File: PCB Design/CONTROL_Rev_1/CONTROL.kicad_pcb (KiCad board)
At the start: 2 copper layers, 40 x 80 mm, 50 parts, among them J1 Conn_01x24_Pin, J2 Conn_01x24_Pin, J3 Micro_SD_Card, J4 USB_C_Receptacle_USB2.0_16P, SW1 SW_SPDT, U1 STM32F446RET6, U2 USBLC6-2SC6, Y1 16MHz, Y2 32.768KHz

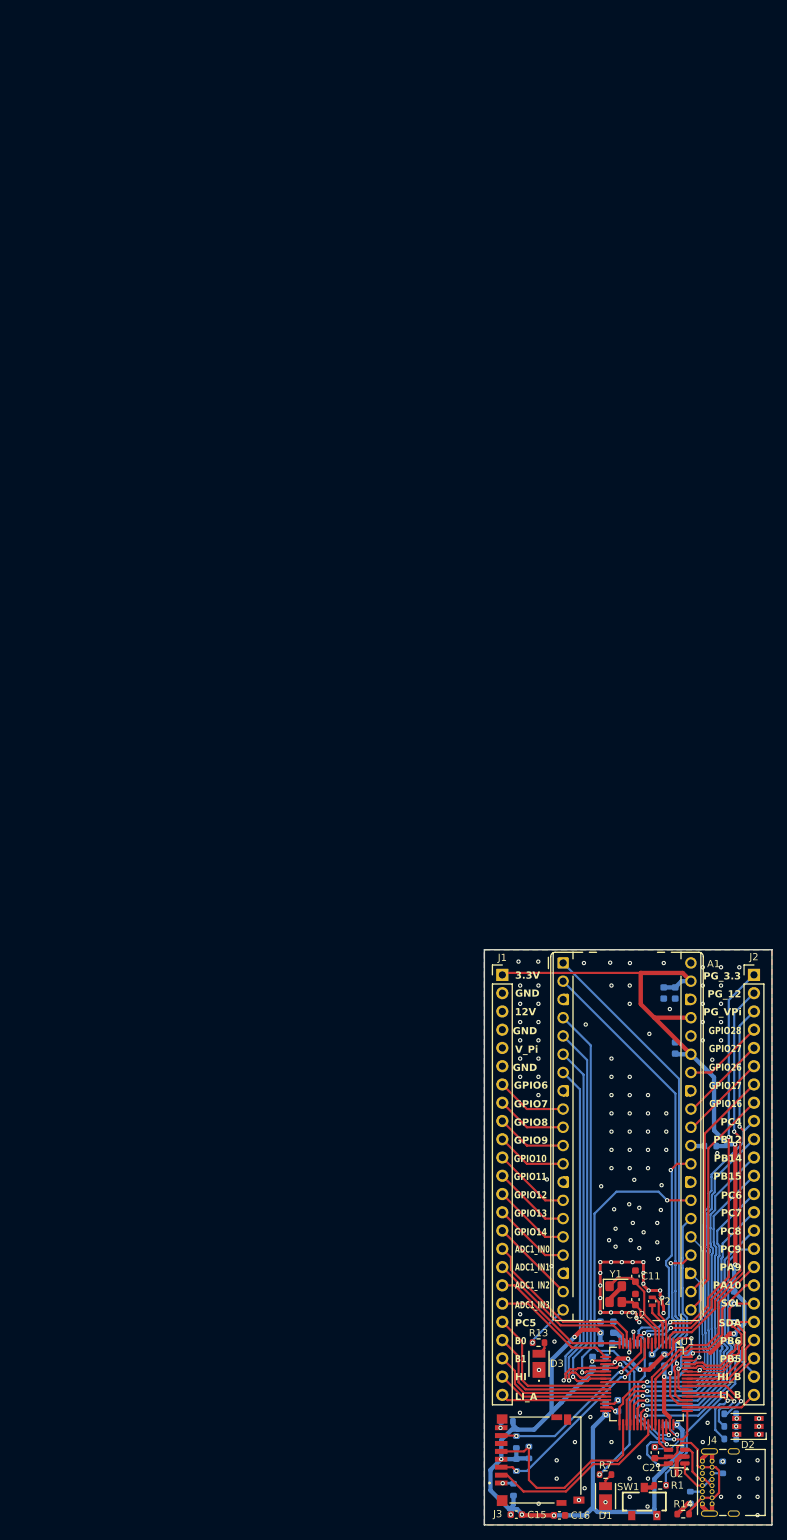
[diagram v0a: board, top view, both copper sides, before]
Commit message: Updated
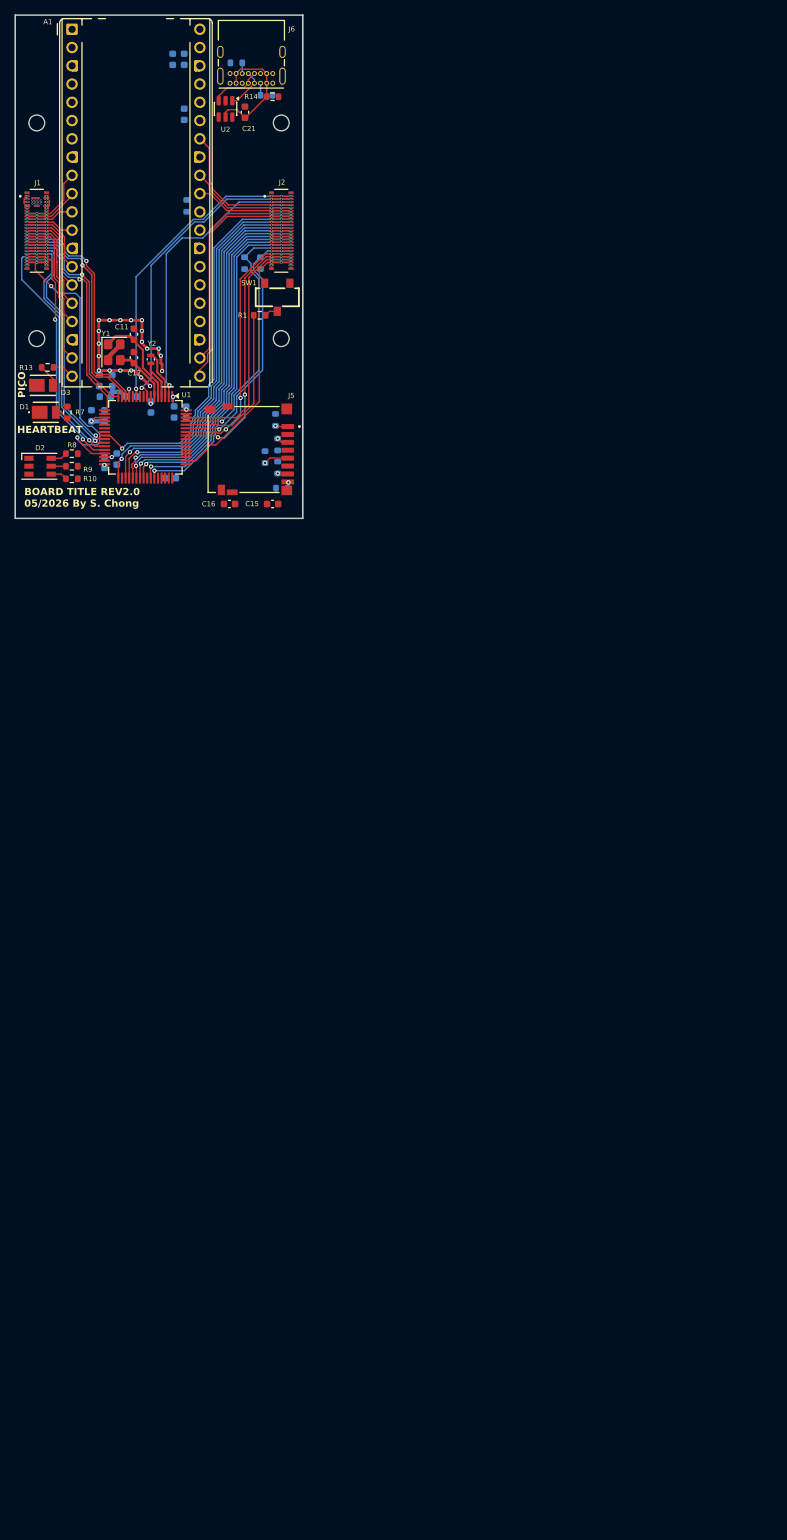
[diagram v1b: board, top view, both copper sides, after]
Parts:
- added J5: Micro_SD_Card, CONTROL:AMPHENOL_1140084168, F.Cu at (17.0, 30.4)
- added J6: USB_C_Receptacle_USB2.0_16P, Connector_USB:USB_C_Receptacle_GCT_USB4085, F.Cu at (15.8, -20.5)
- added REF**: MountingHole_2.2mm_M2, MountingHole:MountingHole_2.2mm_M2, F.Cu at (-17.0, 15.0)
- added REF**: MountingHole_2.2mm_M2, MountingHole:MountingHole_2.2mm_M2, F.Cu at (17.0, 15.0)
- added REF**: MountingHole_2.2mm_M2, MountingHole:MountingHole_2.2mm_M2, F.Cu at (-17.0, -15.0)
- added REF**: MountingHole_2.2mm_M2, MountingHole:MountingHole_2.2mm_M2, F.Cu at (17.0, -15.0)
- J1, J2: value Conn_01x24_Pin -> Conn_02x25_Odd_Even; footprint Connector_PinHeader_2.54mm:PinHeader_1x24_P2.54mm_Vertical -> CONTROL:HIROSE_DF40C-50DP-0.4V_51_
- J3: value Micro_SD_Card -> Conn_02x25_Odd_Even; footprint CONTROL:AMPHENOL_1140084168 -> CONTROL:HIROSE_DF40C-50DP-0.4V_51_; moved to B.Cu
- J4: value USB_C_Receptacle_USB2.0_16P -> Conn_02x25_Odd_Even; footprint Connector_USB:USB_C_Receptacle_GCT_USB4085 -> CONTROL:HIROSE_DF40C-50DP-0.4V_51_; moved to B.Cu
- R10, R8, R9: moved to F.Cu
- moved R12 206.7 mm to (10.8, -23.4), turned to 180 degrees
- moved R14 205.3 mm to (15.8, -18.6), turned to 0 degrees
- moved R11 203.8 mm to (14.9, -18.9), turned to 0 degrees
- moved U2 197.7 mm to (9.25, -16.9), turned to -90 degrees
- moved C21 195.0 mm to (11.9, -16.5)
- moved J4 186.5 mm to (17.0, 0.00), turned to -90 degrees
- moved J3 183.1 mm to (-17.0, 0.00)
- moved SW1 175.1 mm to (16.4, 9.25), turned to 180 degrees
- moved R1 172.0 mm to (14.0, 11.8), turned to 180 degrees
- moved D1 169.7 mm to (-15.8, 25.2), turned to 180 degrees
- moved D2 165.9 mm to (-16.6, 32.8), turned to 0 degrees
- moved R7 165.6 mm to (-12.8, 25.2), turned to 90 degrees
- moved R8 164.8 mm to (-12.1, 31.0), turned to 0 degrees
- moved R3 162.1 mm to (14.1, 4.50)
- moved R9 161.9 mm to (-12.1, 32.8), turned to 0 degrees
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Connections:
- J1 pad 1: 3.3V -> GND
- J1 pad 10: /GPIO_9 -> GND
- J1 pad 11: /GPIO_10 -> GND
- J1 pad 12: /GPIO_11 -> GND
- J1 pad 13: /GPIO_12 -> /GPIO_6
- J1 pad 14: /GPIO_13 -> /GPIO_6
- J1 pad 15: /GPIO_14 -> /GPIO_7
- J1 pad 16: /ADC1_IN0 -> /GPIO_7
- J1 pad 17: /ADC1_IN1 -> /GPIO_8
- J1 pad 18: /ADC1_IN2 -> /GPIO_8
- J1 pad 19: /ADC1_IN3 -> /GPIO_9
- J1 pad 20: /PC5 -> /GPIO_9
- J1 pad 21: /PB0 -> /GPIO_10
- J1 pad 22: /PB1 -> /GPIO_10
- J1 pad 23: /HI_A -> /GPIO_11
- J1 pad 24: /LI_A -> /GPIO_11
- J1 pad 3: 12V -> 3.3V
- J1 pad 4: GND -> 3.3V
- J1 pad 5: V_Piezo -> 3.3V
- J1 pad 6: GND -> 3.3V
- J1 pad 7: /GPIO_6 -> 3.3V
- J1 pad 8: /GPIO_7 -> 3.3V
- J1 pad 9: /GPIO_8 -> GND
- J2 pad 10: /PB12 -> /GPIO_27
- J2 pad 11: /PB14 -> /GPIO_26
- J2 pad 12: /PB15 -> /GPIO_26
- J2 pad 13: /PC6 -> /GPIO_17
- J2 pad 14: /PC7 -> /GPIO_17
- J2 pad 15: /PC8 -> /GPIO_16
- J2 pad 16: /PC9 -> /GPIO_16
- J2 pad 17: /PA9 -> /PC4
- J2 pad 18: /PA10 -> /PC4
- J2 pad 19: /SCL -> /PB12
- J2 pad 2: /PC0 -> /PC3
- J2 pad 20: /SDA -> /PB12
- J2 pad 21: /PB6 -> /PB14
- J2 pad 22: /PB5 -> /PB14
- J2 pad 23: /HI_B -> /PB15
- J2 pad 24: /LI_B -> /PB15
- J2 pad 3: /PC13 -> /PC0
- J2 pad 4: /GPIO_28 -> /PC0
- J2 pad 5: /GPIO_27 -> /PC13
- J2 pad 6: /GPIO_26 -> /PC13
- J2 pad 7: /GPIO_17 -> /GPIO_28
- J2 pad 8: /GPIO_16 -> /GPIO_28
- J2 pad 9: /PC4 -> /GPIO_27
- J3 pad 1: /DAT2 -> GND
- J3 pad 10: (no net) -> GND
- J3 pad 2: /CS -> GND
- J3 pad 3: /SPI2_MOSI -> 3.3V
- J3 pad 5: /SPI2_SCK -> 3.3V
- J3 pad 6: GND -> 3.3V
- J3 pad 7: /SPI2_MISO -> 3.3V
- J3 pad 8: /DAT1 -> 3.3V
- R11 pad 1: Net-(J4-CC1) -> Net-(J6-CC1)
- R12 pad 1: Net-(J4-CC2) -> Net-(J6-CC2)
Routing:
- net 3.3V: track 246.4 -> 6.47 mm, vias 17 -> 18
- net /HEARTBEAT: track 71.6 -> 0.00 mm, vias 3 -> 0
- net /STM_UART_RX: track 69.8 -> 0.00 mm, vias 1 -> 0
- net /STM_UART_TX: track 67.8 -> 0.00 mm, vias 1 -> 0
- net /SWCLK: track 59.1 -> 0.00 mm, vias 2 -> 0
- net GND: track 89.5 -> 33.1 mm, vias 139 -> 30
- net /SPI_SCK: track 54.8 -> 0.00 mm, vias 1 -> 0
- net /SPI_MOSI: track 54.5 -> 0.00 mm, vias 1 -> 0
- net /SPI_MISO: track 53.9 -> 0.00 mm, vias 1 -> 0
- net /SWDIO: track 48.6 -> 0.00 mm, vias 2 -> 0
- net /LI_A: track 14.7 -> 44.6 mm, vias 0 -> 5
- net /LI_B: track 9.99 -> 39.4 mm, vias 0 -> 3
- net /PB5: track 10.6 -> 39.0 mm, vias 0 -> 5
- net /SPI2_MOSI: track 28.7 -> 2.32 mm, vias 2 -> 1
- net /PB6: track 12.5 -> 38.9 mm, vias 0 -> 5
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- added copper zone on B.Cu, net 3.3V
- added copper zone on F.Cu, net 3.3V
- removed copper zone on B.Cu, net GND
- removed copper zone on F.Cu, net GND
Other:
- board size 40 x 80 mm -> 40 x 70 mm
- board text added: "BOARD TITLE REV2.0 05/2026 By S. Chong"
- board text added: "HEARTBEAT"
- board text added: "PICO"
- board text removed: "12V"
- board text removed: "3.3V"
- board text removed: "ADC1_IN0"
- board text removed: "ADC1_IN1"
- board text removed: "ADC1_IN2"
- board text removed: "ADC1_IN3"
- board text removed: "B0"
- board text removed: "B1"
- board text removed: "CONTROL BOARD REV1.1 03/2026 By Samantha Chong"
- board text removed: "GND"
- board text removed: "GPIO10"
- board text removed: "GPIO11"
- board text removed: "GPIO12"
- board text removed: "GPIO13"
- board text removed: "GPIO14"
- board text removed: "GPIO16"
- board text removed: "GPIO17"
- board text removed: "GPIO26"
- board text removed: "GPIO27"
- board text removed: "GPIO28"
- board text removed: "GPIO6"
- board text removed: "GPIO7"
- board text removed: "GPIO8"
- board text removed: "GPIO9"
- board text removed: "HI"
- board text removed: "HI_B"
- board text removed: "LI_A"
- board text removed: "LI_B"
- board text removed: "PA10"
- board text removed: "PA9"
- board text removed: "PB12"
- board text removed: "PB14"
- board text removed: "PB15"
- board text removed: "PB5"
- board text removed: "PB6"
- board text removed: "PC4"
- board text removed: "PC5"
- board text removed: "PC6"
- board text removed: "PC7"
- board text removed: "PC8"
- board text removed: "PC9"
- board text removed: "PG_12"
- board text removed: "PG_3.3"
- board text removed: "PG_VPi"
- board text removed: "SCL"
- board text removed: "SDA"
- board text removed: "V_Pi"

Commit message: Revert "Updated"
This reverts commit 89be44ed720659141c8ee702c54a520a60db740f.
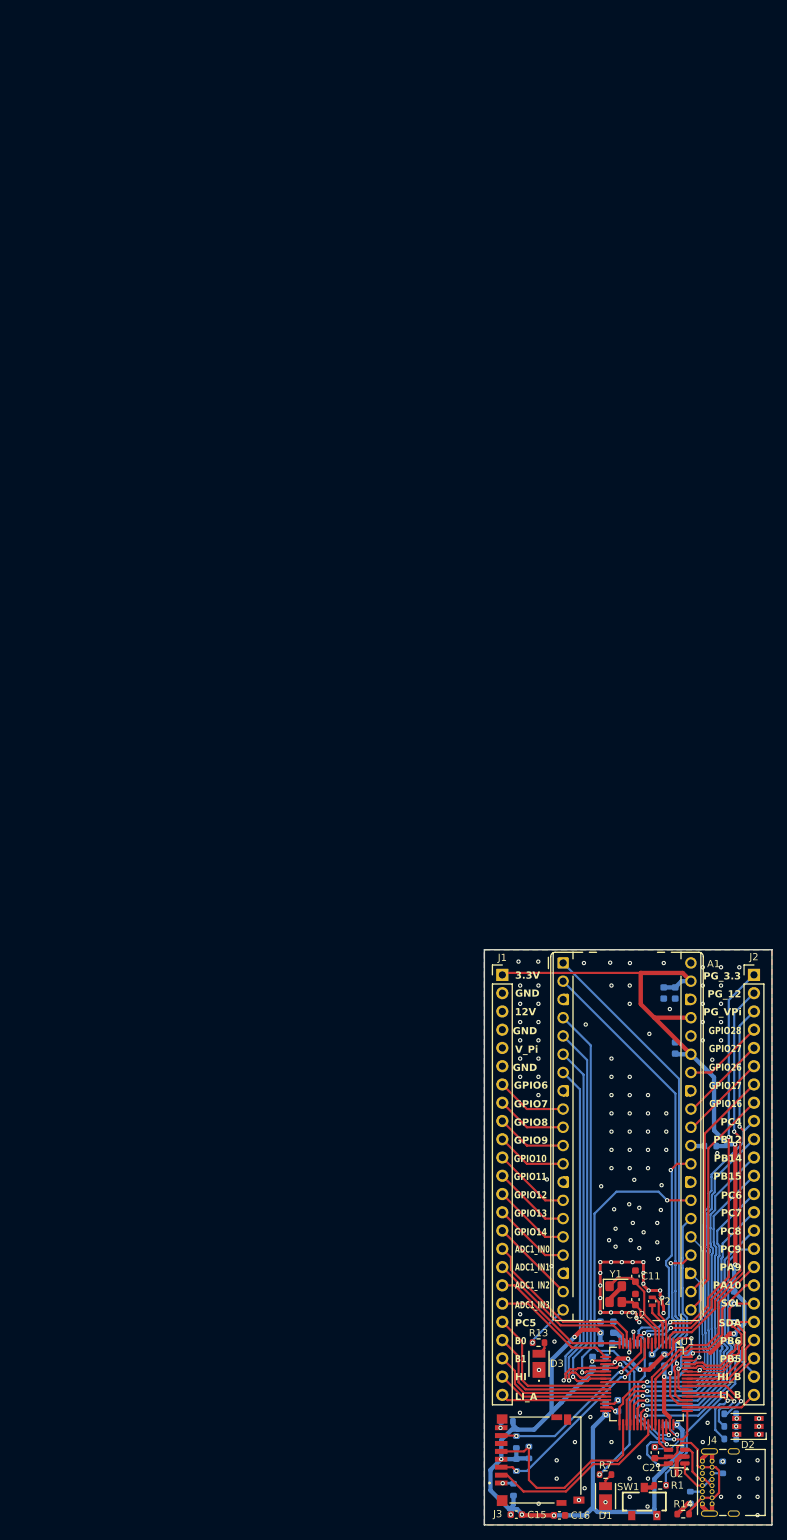
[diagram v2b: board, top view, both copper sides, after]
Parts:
- removed J5: Micro_SD_Card, CONTROL:AMPHENOL_1140084168
- removed J6: USB_C_Receptacle_USB2.0_16P, Connector_USB:USB_C_Receptacle_GCT_USB4085
- removed REF** (x4): MountingHole_2.2mm_M2, MountingHole:MountingHole_2.2mm_M2
- J1, J2: value Conn_02x25_Odd_Even -> Conn_01x24_Pin; footprint CONTROL:HIROSE_DF40C-50DP-0.4V_51_ -> Connector_PinHeader_2.54mm:PinHeader_1x24_P2.54mm_Vertical
- J3: value Conn_02x25_Odd_Even -> Micro_SD_Card; footprint CONTROL:HIROSE_DF40C-50DP-0.4V_51_ -> CONTROL:AMPHENOL_1140084168; moved to F.Cu
- J4: value Conn_02x25_Odd_Even -> USB_C_Receptacle_USB2.0_16P; footprint CONTROL:HIROSE_DF40C-50DP-0.4V_51_ -> Connector_USB:USB_C_Receptacle_GCT_USB4085; moved to F.Cu
- R10, R8, R9: moved to B.Cu
- moved R12 206.7 mm to (78.4, 172.0), turned to 90 degrees
- moved R14 205.3 mm to (72.9, 178.5), turned to 180 degrees
- moved R11 203.8 mm to (73.9, 176.2), turned to -90 degrees
- moved U2 197.7 mm to (72.0, 170.5), turned to 180 degrees
- moved C21 195.0 mm to (69.0, 169.9)
- moved J4 186.5 mm to (75.6, 177.1), turned to 90 degrees
- moved J3 183.1 mm to (48.5, 171.0)
- moved SW1 175.1 mm to (67.5, 176.8), turned to 0 degrees
- moved R1 172.0 mm to (69.7, 174.5), turned to 0 degrees
- moved D1 169.7 mm to (62.1, 176.0), turned to -90 degrees
- moved D2 165.9 mm to (81.9, 166.3), turned to 180 degrees
- moved R7 165.6 mm to (62.1, 173.0), turned to 180 degrees
- moved R8 164.8 mm to (79.5, 168.1), turned to 180 degrees
- moved R3 162.1 mm to (80.0, 152.6)
- moved R9 161.9 mm to (79.5, 166.3), turned to 180 degrees
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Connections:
- J1 pad 1: GND -> 3.3V
- J1 pad 10: GND -> /GPIO_9
- J1 pad 11: GND -> /GPIO_10
- J1 pad 12: GND -> /GPIO_11
- J1 pad 13: /GPIO_6 -> /GPIO_12
- J1 pad 14: /GPIO_6 -> /GPIO_13
- J1 pad 15: /GPIO_7 -> /GPIO_14
- J1 pad 16: /GPIO_7 -> /ADC1_IN0
- J1 pad 17: /GPIO_8 -> /ADC1_IN1
- J1 pad 18: /GPIO_8 -> /ADC1_IN2
- J1 pad 19: /GPIO_9 -> /ADC1_IN3
- J1 pad 20: /GPIO_9 -> /PC5
- J1 pad 21: /GPIO_10 -> /PB0
- J1 pad 22: /GPIO_10 -> /PB1
- J1 pad 23: /GPIO_11 -> /HI_A
- J1 pad 24: /GPIO_11 -> /LI_A
- J1 pad 3: 3.3V -> 12V
- J1 pad 4: 3.3V -> GND
- J1 pad 5: 3.3V -> V_Piezo
- J1 pad 6: 3.3V -> GND
- J1 pad 7: 3.3V -> /GPIO_6
- J1 pad 8: 3.3V -> /GPIO_7
- J1 pad 9: GND -> /GPIO_8
- J2 pad 10: /GPIO_27 -> /PB12
- J2 pad 11: /GPIO_26 -> /PB14
- J2 pad 12: /GPIO_26 -> /PB15
- J2 pad 13: /GPIO_17 -> /PC6
- J2 pad 14: /GPIO_17 -> /PC7
- J2 pad 15: /GPIO_16 -> /PC8
- J2 pad 16: /GPIO_16 -> /PC9
- J2 pad 17: /PC4 -> /PA9
- J2 pad 18: /PC4 -> /PA10
- J2 pad 19: /PB12 -> /SCL
- J2 pad 2: /PC3 -> /PC0
- J2 pad 20: /PB12 -> /SDA
- J2 pad 21: /PB14 -> /PB6
- J2 pad 22: /PB14 -> /PB5
- J2 pad 23: /PB15 -> /HI_B
- J2 pad 24: /PB15 -> /LI_B
- J2 pad 3: /PC0 -> /PC13
- J2 pad 4: /PC0 -> /GPIO_28
- J2 pad 5: /PC13 -> /GPIO_27
- J2 pad 6: /PC13 -> /GPIO_26
- J2 pad 7: /GPIO_28 -> /GPIO_17
- J2 pad 8: /GPIO_28 -> /GPIO_16
- J2 pad 9: /GPIO_27 -> /PC4
- J3 pad 1: GND -> /DAT2
- J3 pad 10: GND -> (no net)
- J3 pad 2: GND -> /CS
- J3 pad 3: 3.3V -> /SPI2_MOSI
- J3 pad 5: 3.3V -> /SPI2_SCK
- J3 pad 6: 3.3V -> GND
- J3 pad 7: 3.3V -> /SPI2_MISO
- J3 pad 8: 3.3V -> /DAT1
- R11 pad 1: Net-(J6-CC1) -> Net-(J4-CC1)
- R12 pad 1: Net-(J6-CC2) -> Net-(J4-CC2)
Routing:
- net 3.3V: track 6.47 -> 246.4 mm, vias 18 -> 17
- net /HEARTBEAT: track 0.00 -> 71.6 mm, vias 0 -> 3
- net /STM_UART_RX: track 0.00 -> 69.8 mm, vias 0 -> 1
- net /STM_UART_TX: track 0.00 -> 67.8 mm, vias 0 -> 1
- net /SWCLK: track 0.00 -> 59.1 mm, vias 0 -> 2
- net GND: track 33.1 -> 89.5 mm, vias 30 -> 139
- net /SPI_SCK: track 0.00 -> 54.8 mm, vias 0 -> 1
- net /SPI_MOSI: track 0.00 -> 54.5 mm, vias 0 -> 1
- net /SPI_MISO: track 0.00 -> 53.9 mm, vias 0 -> 1
- net /SWDIO: track 0.00 -> 48.6 mm, vias 0 -> 2
- net /LI_A: track 44.6 -> 14.7 mm, vias 5 -> 0
- net /LI_B: track 39.4 -> 9.99 mm, vias 3 -> 0
- net /PB5: track 39.0 -> 10.6 mm, vias 5 -> 0
- net /SPI2_MOSI: track 2.32 -> 28.7 mm, vias 1 -> 2
- net /PB6: track 38.9 -> 12.5 mm, vias 5 -> 0
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- added copper zone on B.Cu, net GND
- added copper zone on F.Cu, net GND
- removed copper zone on B.Cu, net 3.3V
- removed copper zone on F.Cu, net 3.3V
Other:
- board size 40 x 70 mm -> 40 x 80 mm
- board text added: "12V"
- board text added: "3.3V"
- board text added: "ADC1_IN0"
- board text added: "ADC1_IN1"
- board text added: "ADC1_IN2"
- board text added: "ADC1_IN3"
- board text added: "B0"
- board text added: "B1"
- board text added: "CONTROL BOARD REV1.1 03/2026 By Samantha Chong"
- board text added: "GND"
- board text added: "GPIO10"
- board text added: "GPIO11"
- board text added: "GPIO12"
- board text added: "GPIO13"
- board text added: "GPIO14"
- board text added: "GPIO16"
- board text added: "GPIO17"
- board text added: "GPIO26"
- board text added: "GPIO27"
- board text added: "GPIO28"
- board text added: "GPIO6"
- board text added: "GPIO7"
- board text added: "GPIO8"
- board text added: "GPIO9"
- board text added: "HI"
- board text added: "HI_B"
- board text added: "LI_A"
- board text added: "LI_B"
- board text added: "PA10"
- board text added: "PA9"
- board text added: "PB12"
- board text added: "PB14"
- board text added: "PB15"
- board text added: "PB5"
- board text added: "PB6"
- board text added: "PC4"
- board text added: "PC5"
- board text added: "PC6"
- board text added: "PC7"
- board text added: "PC8"
- board text added: "PC9"
- board text added: "PG_12"
- board text added: "PG_3.3"
- board text added: "PG_VPi"
- board text added: "SCL"
- board text added: "SDA"
- board text added: "V_Pi"
- board text removed: "BOARD TITLE REV2.0 05/2026 By S. Chong"
- board text removed: "HEARTBEAT"
- board text removed: "PICO"
